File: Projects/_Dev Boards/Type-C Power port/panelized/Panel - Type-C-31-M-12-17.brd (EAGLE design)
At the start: 100 x 100 mm, 40 parts, among them J1 USB-TYPE-C-31-M-12, J10 USB-TYPE-C-31-M-17, J11 USB-TYPE-C-31-M-17, J12 USB-TYPE-C-31-M-17, J13 USB-TYPE-C-31-M-17, J14 USB-TYPE-C-31-M-17, J15 USB-TYPE-C-31-M-17, J16 USB-TYPE-C-31-M-12, J17 USB-TYPE-C-31-M-12, J18 USB-TYPE-C-31-M-12, J19 USB-TYPE-C-31-M-12, J2 USB-TYPE-C-31-M-17, J20 USB-TYPE-C-31-M-12, J3 USB-TYPE-C-31-M-12, J4 USB-TYPE-C-31-M-12, J5 USB-TYPE-C-31-M-12, J6 USB-TYPE-C-31-M-12, J7 USB-TYPE-C-31-M-17, J8 USB-TYPE-C-31-M-17, J9 USB-TYPE-C-31-M-17

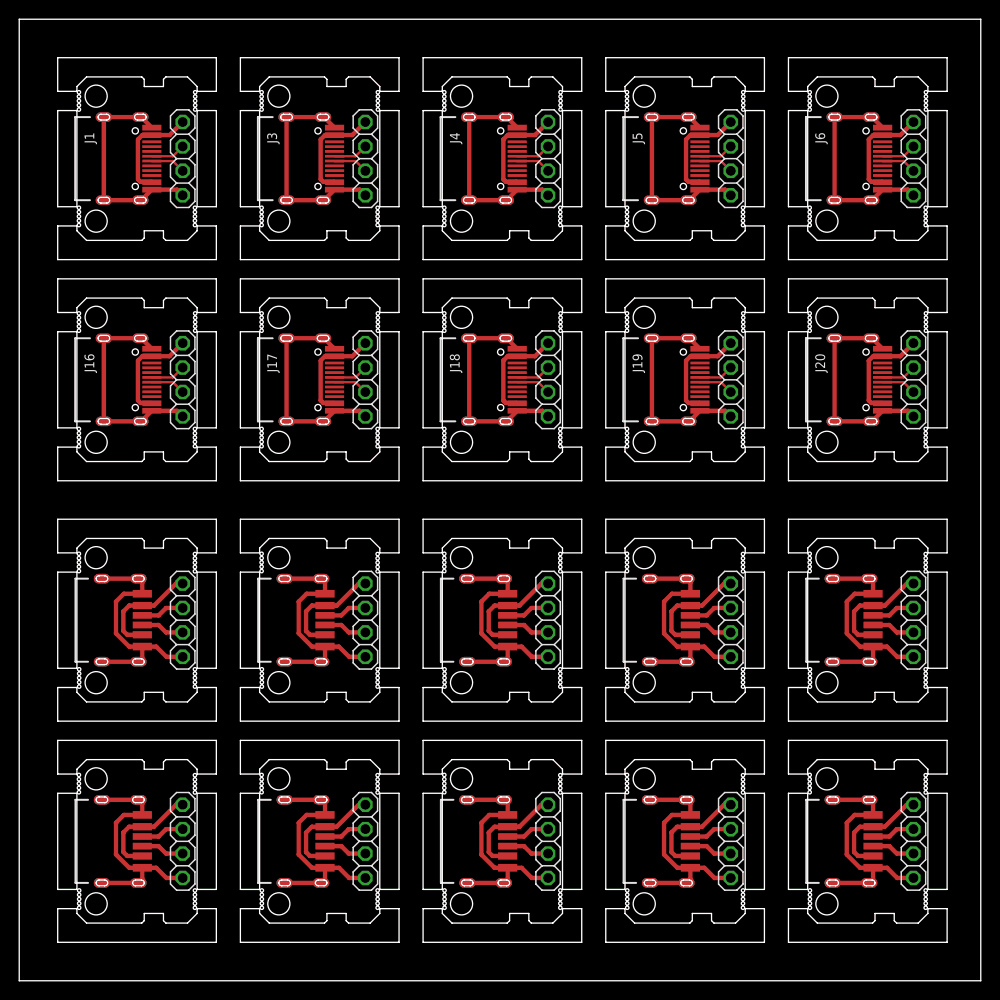
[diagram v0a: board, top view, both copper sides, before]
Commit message: update
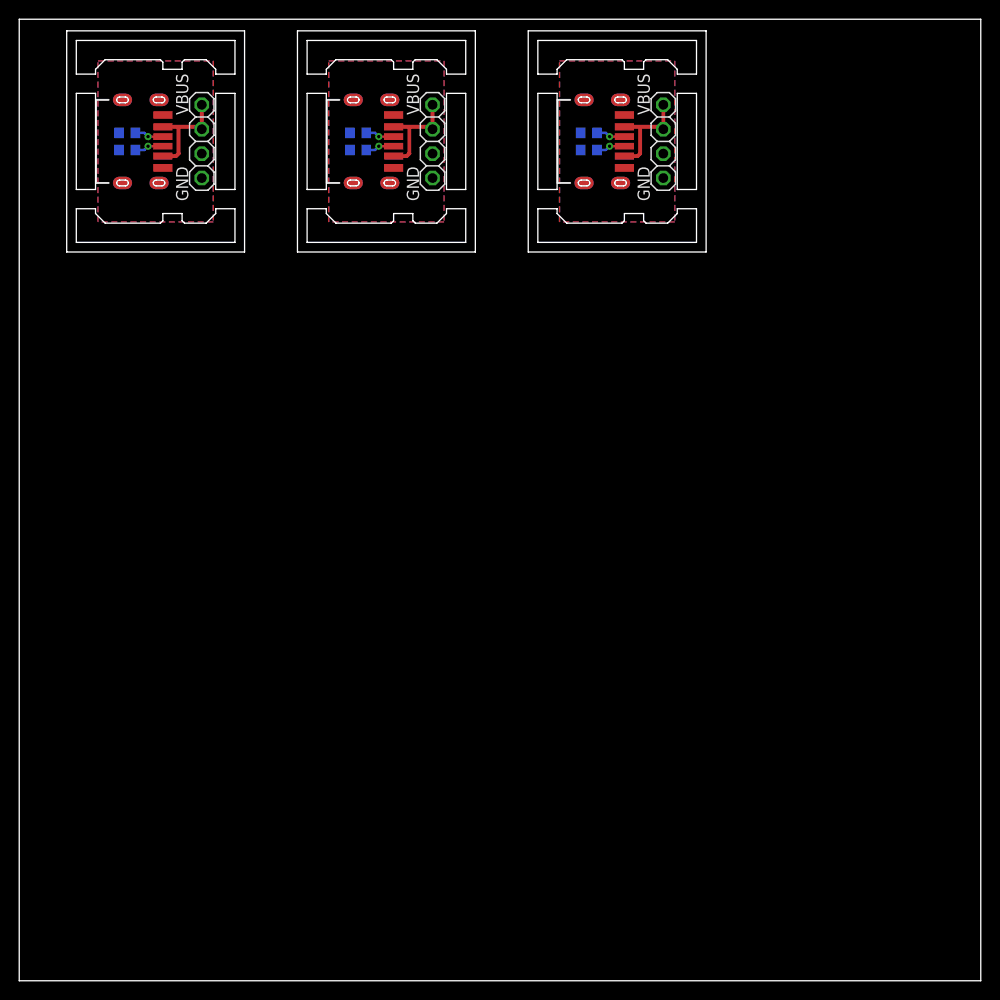
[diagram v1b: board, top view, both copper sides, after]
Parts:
- removed J10, J11, J12, J13, J14, J15, J7, J8, J9: USB-TYPE-C-31-M-17, angrypig7-Connectors:USB-TYPE-C-31-M-17
- removed J16, J17, J18, J19, J20, J4, J5, J6: USB-TYPE-C-31-M-12, angrypig7-Connectors:USB-TYPE-C-31-M-12
- removed JP10, JP11, JP12, JP13, JP14, JP15, JP16, JP17, JP18, JP19, JP20, JP4, JP5, JP6, JP7, JP8, JP9: (no value), pinhead_v2:1X04/OCT
- added R1, R2, R3, R4, R5, R6: 5.1k, angrypig7-RCL:R0603
- J1, J3: value USB-TYPE-C-31-M-12 -> USB-TYPE-C-31-M-17; device angrypig7-Connectors:USB-TYPE-C-31-M-12 -> angrypig7-Connectors:USB-TYPE-C-31-M-17
- JP1, JP2, JP3: device pinhead_v2:1X04/OCT -> angrypig7-Connectors-PinHeads:1X04
- moved J2 77.3 mm to (38.5, 87.3)
- moved JP1 72.8 mm to (19.0, 87.3)
- moved JP3 31.0 mm to (67.0, 87.3)
- moved J3 31.0 mm to (62.5, 87.3)
- moved JP2 26.0 mm to (43.0, 87.3)
- moved J1 2.64 mm to (14.5, 87.3)
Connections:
- removed net N$10: J3.A6, JP3.2
- removed net N$11: J3.A7, JP3.3
- removed net N$12: J3.GND1, J3.GND2, J3.SHLD-B1, J3.SHLD-B2, J3.SHLD-B3, J3.SHLD-B4, J3.SHLD-T1, J3.SHLD-T2, J3.SHLD-T3, J3.SHLD-T4, JP3.4
- removed net N$13: J4.VBUS1, J4.VBUS2, JP4.1
- removed net N$14: J4.A6, JP4.2
- removed net N$15: J4.A7, JP4.3
- removed net N$16: J4.GND1, J4.GND2, J4.SHLD-B1, J4.SHLD-B2, J4.SHLD-B3, J4.SHLD-B4, J4.SHLD-T1, J4.SHLD-T2, J4.SHLD-T3, J4.SHLD-T4, JP4.4
- removed net N$17: J5.VBUS1, J5.VBUS2, JP5.1
- removed net N$18: J5.A6, JP5.2
- removed net N$19: J5.A7, JP5.3
- removed net N$20: J5.GND1, J5.GND2, J5.SHLD-B1, J5.SHLD-B2, J5.SHLD-B3, J5.SHLD-B4, J5.SHLD-T1, J5.SHLD-T2, J5.SHLD-T3, J5.SHLD-T4, JP5.4
- removed net N$21: J6.VBUS1, J6.VBUS2, JP6.1
- removed net N$22: J6.A6, JP6.2
- removed net N$23: J6.A7, JP6.3
- removed net N$24: J6.GND1, J6.GND2, J6.SHLD-B1, J6.SHLD-B2, J6.SHLD-B3, J6.SHLD-B4, J6.SHLD-T1, J6.SHLD-T2, J6.SHLD-T3, J6.SHLD-T4, JP6.4
- removed net N$25: J7.GND, J7.GND_2, J7.SHLD-B1, J7.SHLD-B2, J7.SHLD-B3, J7.SHLD-B4, J7.SHLD-T1, J7.SHLD-T2, J7.SHLD-T3, J7.SHLD-T4, JP7.4
- removed net N$26: J7.VBUS, J7.VBUS_2, JP7.1
- removed net N$27: J7.CC1, JP7.2
- removed net N$28: J7.CC2, JP7.3
- removed net N$29: J8.GND, J8.GND_2, J8.SHLD-B1, J8.SHLD-B2, J8.SHLD-B3, J8.SHLD-B4, J8.SHLD-T1, J8.SHLD-T2, J8.SHLD-T3, J8.SHLD-T4, JP8.4
- removed net N$30: J8.VBUS, J8.VBUS_2, JP8.1
- removed net N$31: J8.CC1, JP8.2
- removed net N$32: J8.CC2, JP8.3
- removed net N$33: J9.GND, J9.GND_2, J9.SHLD-B1, J9.SHLD-B2, J9.SHLD-B3, J9.SHLD-B4, J9.SHLD-T1, J9.SHLD-T2, J9.SHLD-T3, J9.SHLD-T4, JP9.4
- removed net N$34: J9.VBUS, J9.VBUS_2, JP9.1
- removed net N$35: J9.CC1, JP9.2
- removed net N$36: J9.CC2, JP9.3
- removed net N$37: J10.GND, J10.GND_2, J10.SHLD-B1, J10.SHLD-B2, J10.SHLD-B3, J10.SHLD-B4, J10.SHLD-T1, J10.SHLD-T2, J10.SHLD-T3, J10.SHLD-T4, JP10.4
- removed net N$38: J10.VBUS, J10.VBUS_2, JP10.1
- removed net N$39: J10.CC1, JP10.2
- removed net N$40: J10.CC2, JP10.3
- removed net N$41: J11.GND, J11.GND_2, J11.SHLD-B1, J11.SHLD-B2, J11.SHLD-B3, J11.SHLD-B4, J11.SHLD-T1, J11.SHLD-T2, J11.SHLD-T3, J11.SHLD-T4, JP11.4
- removed net N$42: J11.VBUS, J11.VBUS_2, JP11.1
- removed net N$43: J11.CC1, JP11.2
- removed net N$44: J11.CC2, JP11.3
- removed net N$45: J12.GND, J12.GND_2, J12.SHLD-B1, J12.SHLD-B2, J12.SHLD-B3, J12.SHLD-B4, J12.SHLD-T1, J12.SHLD-T2, J12.SHLD-T3, J12.SHLD-T4, JP12.4
- removed net N$46: J12.VBUS, J12.VBUS_2, JP12.1
- removed net N$47: J12.CC1, JP12.2
- removed net N$48: J12.CC2, JP12.3
- removed net N$49: J13.GND, J13.GND_2, J13.SHLD-B1, J13.SHLD-B2, J13.SHLD-B3, J13.SHLD-B4, J13.SHLD-T1, J13.SHLD-T2, J13.SHLD-T3, J13.SHLD-T4, JP13.4
- removed net N$50: J13.VBUS, J13.VBUS_2, JP13.1
- removed net N$51: J13.CC1, JP13.2
- removed net N$52: J13.CC2, JP13.3
- removed net N$53: J14.GND, J14.GND_2, J14.SHLD-B1, J14.SHLD-B2, J14.SHLD-B3, J14.SHLD-B4, J14.SHLD-T1, J14.SHLD-T2, J14.SHLD-T3, J14.SHLD-T4, JP14.4
- removed net N$54: J14.VBUS, J14.VBUS_2, JP14.1
- removed net N$55: J14.CC1, JP14.2
- removed net N$56: J14.CC2, JP14.3
- removed net N$57: J15.GND, J15.GND_2, J15.SHLD-B1, J15.SHLD-B2, J15.SHLD-B3, J15.SHLD-B4, J15.SHLD-T1, J15.SHLD-T2, J15.SHLD-T3, J15.SHLD-T4, JP15.4
- removed net N$58: J15.VBUS, J15.VBUS_2, JP15.1
- removed net N$59: J15.CC1, JP15.2
- removed net N$60: J15.CC2, JP15.3
- removed net N$61: J16.VBUS1, J16.VBUS2, JP16.1
- removed net N$62: J16.A6, JP16.2
- removed net N$63: J16.A7, JP16.3
- removed net N$64: J16.GND1, J16.GND2, J16.SHLD-B1, J16.SHLD-B2, J16.SHLD-B3, J16.SHLD-B4, J16.SHLD-T1, J16.SHLD-T2, J16.SHLD-T3, J16.SHLD-T4, JP16.4
- removed net N$65: J17.VBUS1, J17.VBUS2, JP17.1
- removed net N$66: J17.A6, JP17.2
- removed net N$67: J17.A7, JP17.3
- removed net N$68: J17.GND1, J17.GND2, J17.SHLD-B1, J17.SHLD-B2, J17.SHLD-B3, J17.SHLD-B4, J17.SHLD-T1, J17.SHLD-T2, J17.SHLD-T3, J17.SHLD-T4, JP17.4
- removed net N$69: J18.VBUS1, J18.VBUS2, JP18.1
- removed net N$7: J2.CC1, JP1.2
- removed net N$70: J18.A6, JP18.2
- removed net N$71: J18.A7, JP18.3
- removed net N$72: J18.GND1, J18.GND2, J18.SHLD-B1, J18.SHLD-B2, J18.SHLD-B3, J18.SHLD-B4, J18.SHLD-T1, J18.SHLD-T2, J18.SHLD-T3, J18.SHLD-T4, JP18.4
- removed net N$73: J19.VBUS1, J19.VBUS2, JP19.1
- removed net N$74: J19.A6, JP19.2
- removed net N$75: J19.A7, JP19.3
- removed net N$76: J19.GND1, J19.GND2, J19.SHLD-B1, J19.SHLD-B2, J19.SHLD-B3, J19.SHLD-B4, J19.SHLD-T1, J19.SHLD-T2, J19.SHLD-T3, J19.SHLD-T4, JP19.4
- removed net N$77: J20.VBUS1, J20.VBUS2, JP20.1
- removed net N$78: J20.A6, JP20.2
- removed net N$79: J20.A7, JP20.3
- removed net N$8: J2.CC2, JP1.3
- removed net N$80: J20.GND1, J20.GND2, J20.SHLD-B1, J20.SHLD-B2, J20.SHLD-B3, J20.SHLD-B4, J20.SHLD-T1, J20.SHLD-T2, J20.SHLD-T3, J20.SHLD-T4, JP20.4
- removed net N$9: J3.VBUS1, J3.VBUS2, JP3.1
- new net GND: J1.GND, J1.GND_2, J1.SHLD-B1, J1.SHLD-B2, J1.SHLD-B3, J1.SHLD-B4, J1.SHLD-T1, J1.SHLD-T2, J1.SHLD-T3, J1.SHLD-T4, JP1.3, JP1.4, R1.2, R2.2
- new net GND1: J2.GND, J2.GND_2, J2.SHLD-B1, J2.SHLD-B2, J2.SHLD-B3, J2.SHLD-B4, J2.SHLD-T1, J2.SHLD-T2, J2.SHLD-T3, J2.SHLD-T4, JP2.3, JP2.4, R3.2, R4.2
- new net GND2: J3.GND, J3.GND_2, J3.SHLD-B1, J3.SHLD-B2, J3.SHLD-B3, J3.SHLD-B4, J3.SHLD-T1, J3.SHLD-T2, J3.SHLD-T3, J3.SHLD-T4, JP3.3, JP3.4, R5.2, R6.2
- new net VBUS: J1.VBUS, J1.VBUS_2, JP1.1, JP1.2
- new net VBUS1: J2.VBUS, J2.VBUS_2, JP2.1, JP2.2
- new net VBUS2: J3.VBUS, J3.VBUS_2, JP3.1, JP3.2
- net N$1: now also J1.CC1, R1.1; no longer J1.VBUS1, J1.VBUS2, JP2.1
- net N$2: now also J1.CC2, R2.1; no longer J1.A6, JP2.2
- net N$3: now also J2.CC1, R3.1; no longer J1.A7, JP2.3
- net N$4: now also J2.CC2, R4.1; no longer J1.GND1, J1.GND2, J1.SHLD-B1, J1.SHLD-B2, J1.SHLD-B3, J1.SHLD-B4, J1.SHLD-T1, J1.SHLD-T2, J1.SHLD-T3, J1.SHLD-T4, JP2.4
- net N$5: now also J3.CC1, R5.1; no longer J2.GND, J2.GND_2, J2.SHLD-B1, J2.SHLD-B2, J2.SHLD-B3, J2.SHLD-B4, J2.SHLD-T1, J2.SHLD-T2, J2.SHLD-T3, J2.SHLD-T4, JP1.4
- net N$6: now also J3.CC2, R6.1; no longer J2.VBUS, J2.VBUS_2, JP1.1
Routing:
- net N$57: track 25.4 -> 0.00 mm
- net N$53: track 25.4 -> 0.00 mm
- net N$37: track 25.4 -> 0.00 mm
- net N$33: track 25.4 -> 0.00 mm
- net N$41: track 25.4 -> 0.00 mm
- net N$45: track 25.4 -> 0.00 mm
- net N$25: track 25.4 -> 0.00 mm
- net N$49: track 25.4 -> 0.00 mm
- net N$29: track 25.4 -> 0.00 mm
- net N$80: track 23.0 -> 0.00 mm
- net N$76: track 23.0 -> 0.00 mm
- net N$72: track 23.0 -> 0.00 mm
- net N$24: track 23.0 -> 0.00 mm
- net N$20: track 23.0 -> 0.00 mm
- net N$16: track 23.0 -> 0.00 mm
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- added copper zone on layer 1, net GND
- added copper zone on layer 16, net GND
- added copper zone on layer 1, net GND1
- added copper zone on layer 16, net GND1
- added copper zone on layer 1, net GND2
- added copper zone on layer 16, net GND2
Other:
- outline, holes or cut-outs redrawn
- board text removed: "CC1"
- board text removed: "CC2"
- board text removed: "D+"
- board text removed: "D-"
